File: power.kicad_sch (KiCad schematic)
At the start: 19 parts, among them J201 Conn_01x02, J202 Conn_01x04, J203 Conn_01x04, J204 Conn_01x04, SW201 SW_DPDT_x2, U201 AZ1117CH2-5.0TRG1, U202 MIC5317-3.3YM5-TR

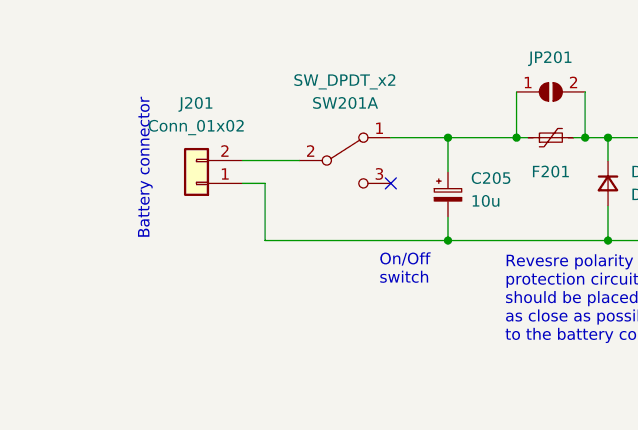
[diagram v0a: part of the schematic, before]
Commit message: Prof approved commit
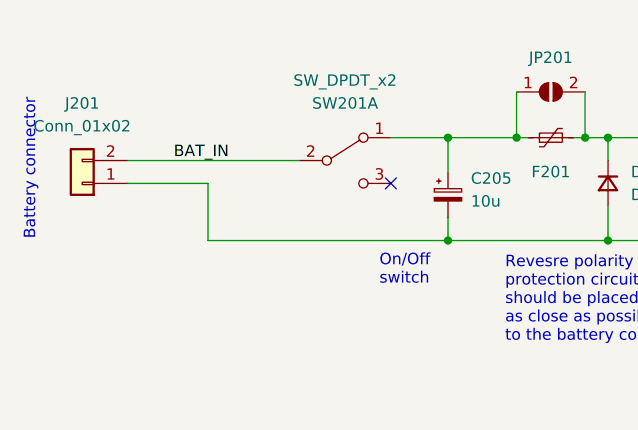
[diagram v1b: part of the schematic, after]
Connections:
- net BAT_IN: now reaches J201.2 (Pin_2), SW201.2 (B)
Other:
- moved on the sheet: J201
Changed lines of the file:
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@@
     (stroke (width 0) (type default) (color 0 0 0 0))
   )
-  (wire (pts (xy 110.49 133.35) (xy 107.95 133.35))
+  (wire (pts (xy 104.14 133.35) (xy 95.25 133.35))
     (stroke (width 0) (type default) (color 0 0 0 0))
   )
@@
     (stroke (width 0) (type default) (color 0 0 0 0))
   )
-  (wire (pts (xy 107.95 130.81) (xy 114.3 130.81))
+  (wire (pts (xy 95.25 130.81) (xy 114.3 130.81))
     (stroke (width 0) (type default) (color 0 0 0 0))
   )
@@
     (stroke (width 0) (type default) (color 0 0 0 0))
   )
-  (wire (pts (xy 110.49 139.7) (xy 110.49 133.35))
+  (wire (pts (xy 104.14 139.7) (xy 104.14 133.35))
     (stroke (width 0) (type default) (color 0 0 0 0))
   )
@@
     (stroke (width 0) (type default) (color 0 0 0 0))
   )
-  (wire (pts (xy 110.49 139.7) (xy 130.81 139.7))
+  (wire (pts (xy 104.14 139.7) (xy 130.81 139.7))
     (stroke (width 0) (type default) (color 0 0 0 0))
   )
@@
     (effects (font (size 1.27 1.27)) (justify left bottom))
   )
-  (text "Battery connector" (at 97.79 139.7 90)
+  (text "Battery connector" (at 85.09 139.7 90)
     (effects (font (size 1.27 1.27)) (justify left bottom))
   )
   (text "5V regulator" (at 212.09 123.19 0)
+    (effects (font (size 1.27 1.27)) (justify left bottom))
+  )
+  (label "BAT_IN" (at 100.33 130.81 0)
     (effects (font (size 1.27 1.27)) (justify left bottom))
   )
@@
     (pin "2")
   )
-  (symbol (lib_id "Connector_Generic:Conn_01x02") (at 102.87 133.35 180) (unit 1)
-    (in_bom yes) (on_board yes) (fields_autoplaced)
-    (property "Reference" "J201" (id 0) (at 102.87 124.46 0))
-    (property "Value" "Conn_01x02" (id 1) (at 102.87 127 0))
-    (property "Footprint" "Connector_JST:JST_XH_B2B-XH-A_1x02_P2.50mm_Vertical" (id 2) (at 102.87 133.35 0)
-      (effects (font (size 1.27 1.27)) hide)
-    )
-    (property "Datasheet" "~" (id 3) (at 102.87 133.35 0)
-      (effects (font (size 1.27 1.27)) hide)
-    )
+  (symbol (lib_id "Connector_Generic:Conn_01x02") (at 90.17 133.35 180) (unit 1)
+    (in_bom yes) (on_board yes) (fields_autoplaced)
+    (property "Reference" "J201" (id 0) (at 90.17 124.46 0))
+    (property "Value" "Conn_01x02" (id 1) (at 90.17 127 0))
+    (property "Footprint" "Connector_JST:JST_XH_B2B-XH-A_1x02_P2.50mm_Vertical" (id 2) (at 90.17 133.35 0)
+      (effects (font (size 1.27 1.27)) hide)
+    )
+    (property "Datasheet" "~" (id 3) (at 90.17 133.35 0)
+      (effects (font (size 1.27 1.27)) hide)
+    )
